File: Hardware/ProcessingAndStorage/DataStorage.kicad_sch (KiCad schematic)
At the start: 10 parts, among them J3 SD_Card_Receptacle, U3 LD1117S50TR_SOT223

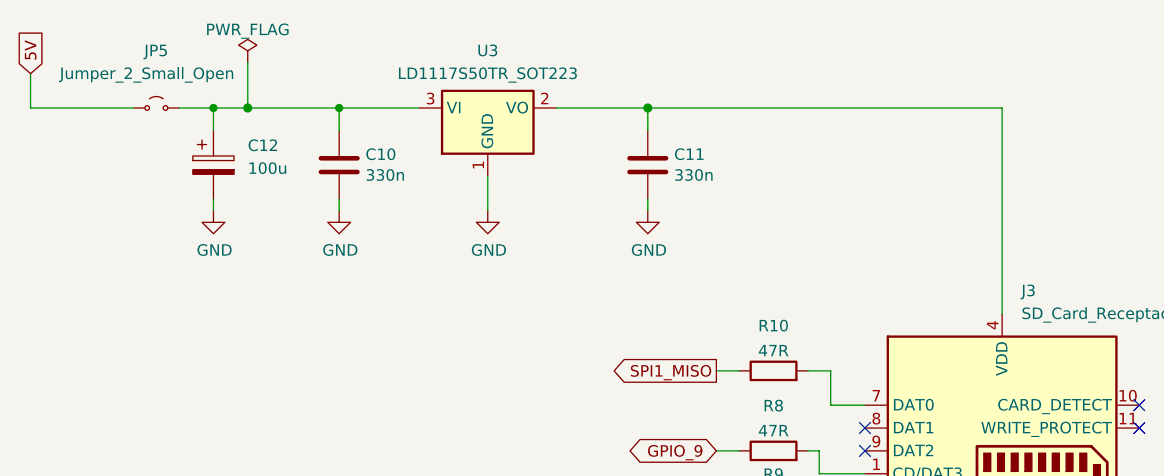
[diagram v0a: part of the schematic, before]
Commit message: make hw
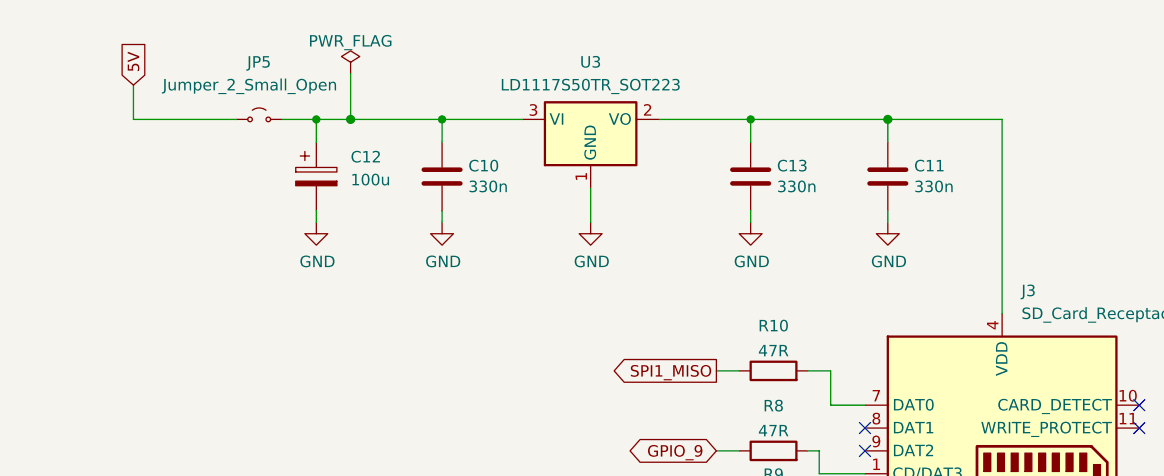
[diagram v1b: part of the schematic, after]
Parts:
- added C13: 330n, Capacitor_SMD:C_0805_2012Metric, symbol Device:C
- J3: footprint (none) -> Connector_Card:SD_TE_2041021
- U3: footprint Package_TO_SOT_SMD:SOT-223 -> Package_TO_SOT_SMD:SOT-223-3_TabPin2
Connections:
- net GND: now also C13.2
- net at C11.1, J3.4 (VDD), U3.2 (VO): now also C13.1
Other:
- moved on the sheet: C10, C11, C12, JP5, U3
